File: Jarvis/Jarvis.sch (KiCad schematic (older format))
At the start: 180 parts, among them IC1 ADP1607, IC2 MAX-8Q, IC3 MPU-9250, IC4 STM32F411CxUx, IC5 Si4460, IC6 MS5611-01BA03, IC7 S25FL127S, J1 PYRO, J2 PWR, J3 ARM, J4 MICROUSB, P1 SMA, P2 SMA, P3 SWD_TC, Q1 PFET, Q2 PFET, Q3 PFET, Q4 NFET, Q5 NFET, Q6 NFET, Q7 NFET, X1 434MHz ANT, X10 Housing x1, X11 Housing x3, X12 M Crimps x6, X13 F Crimps x17, X14 Crimp Tool, X15 RF Frame, X16 RF Cover, X2 Red LED, X3 AA Battery, X4 AA Holder, X5 ARM Switch, X6 Wire, X7 Heat Shrink, X8 Housing x1, X9 Housing x4, Y1 26MHz, Y2 30MHz

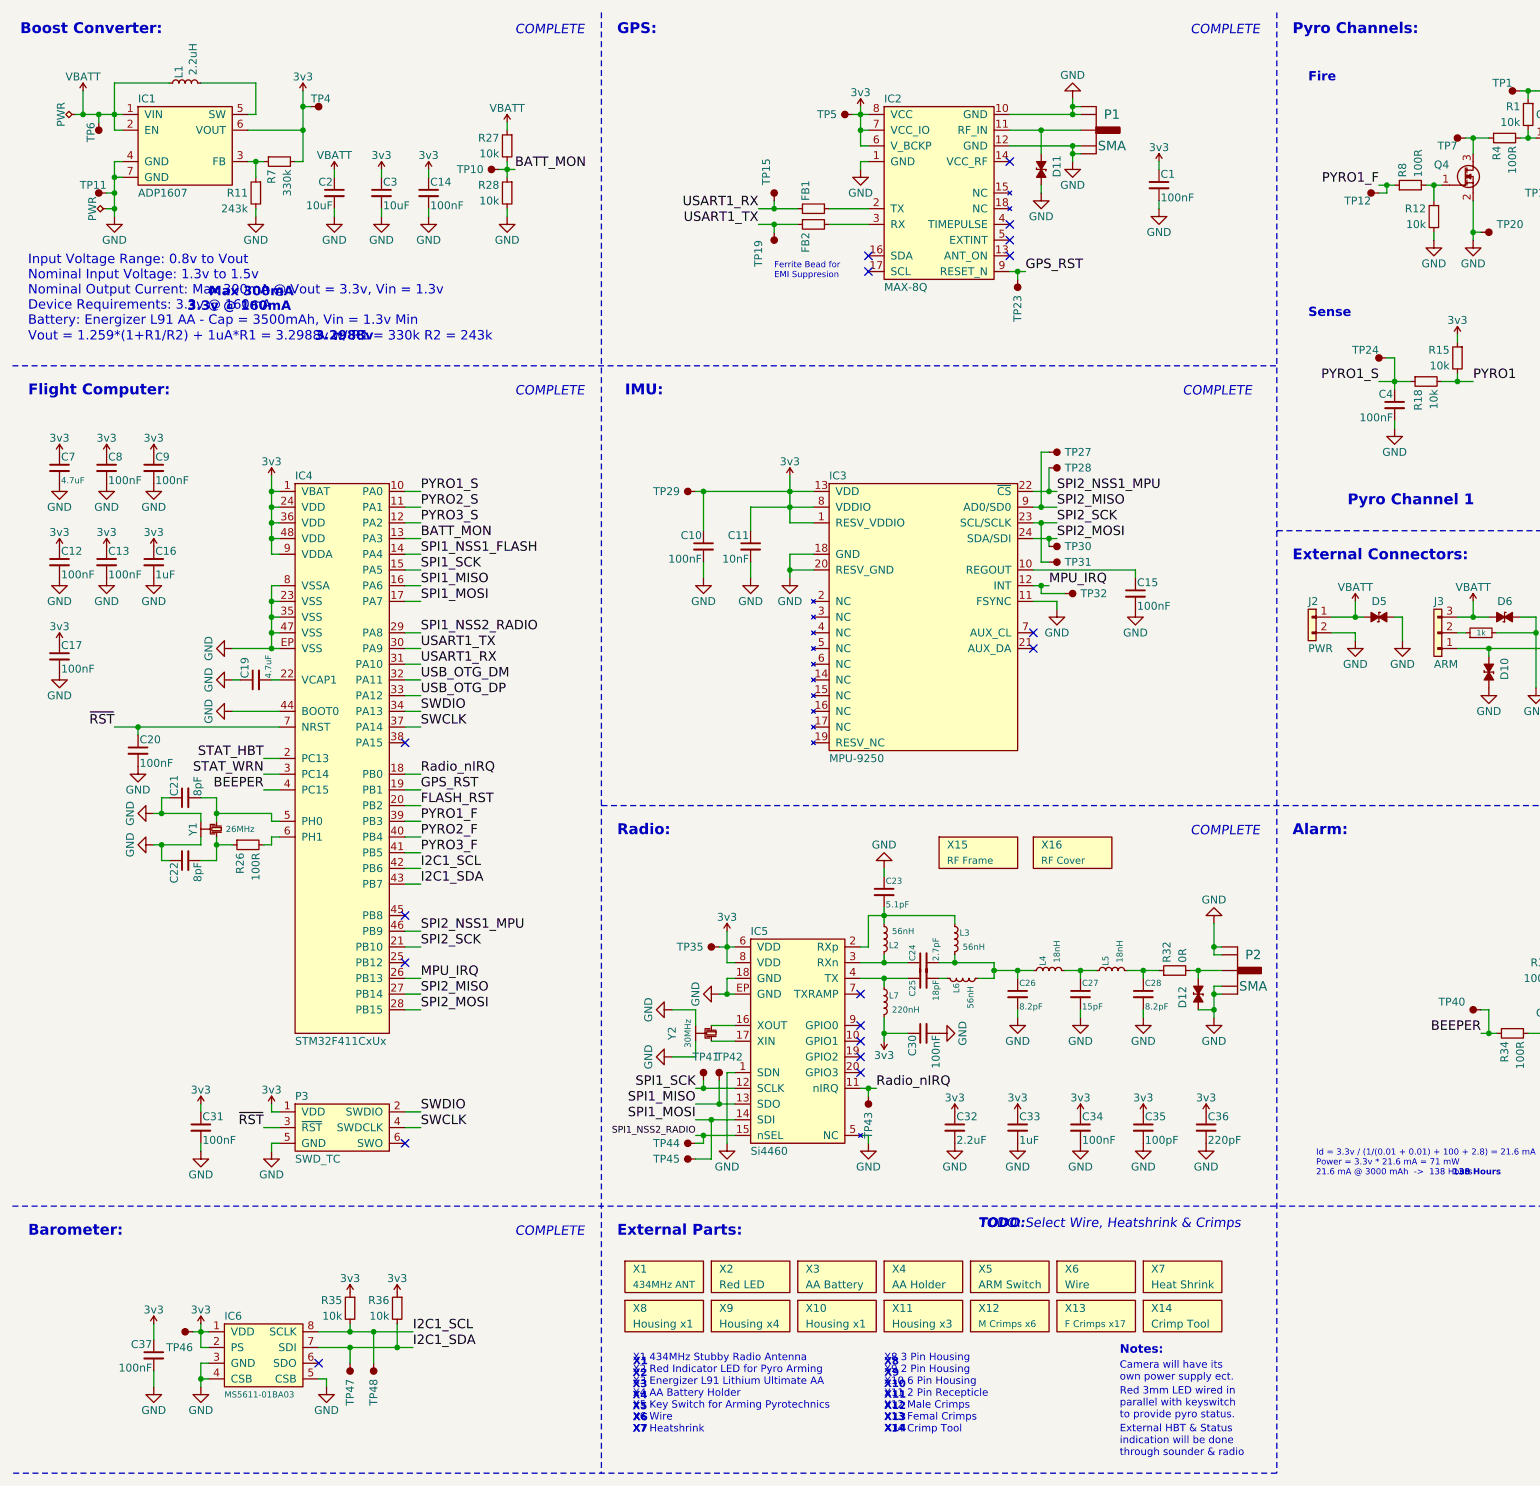
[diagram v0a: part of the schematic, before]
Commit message: Checked all Footprints
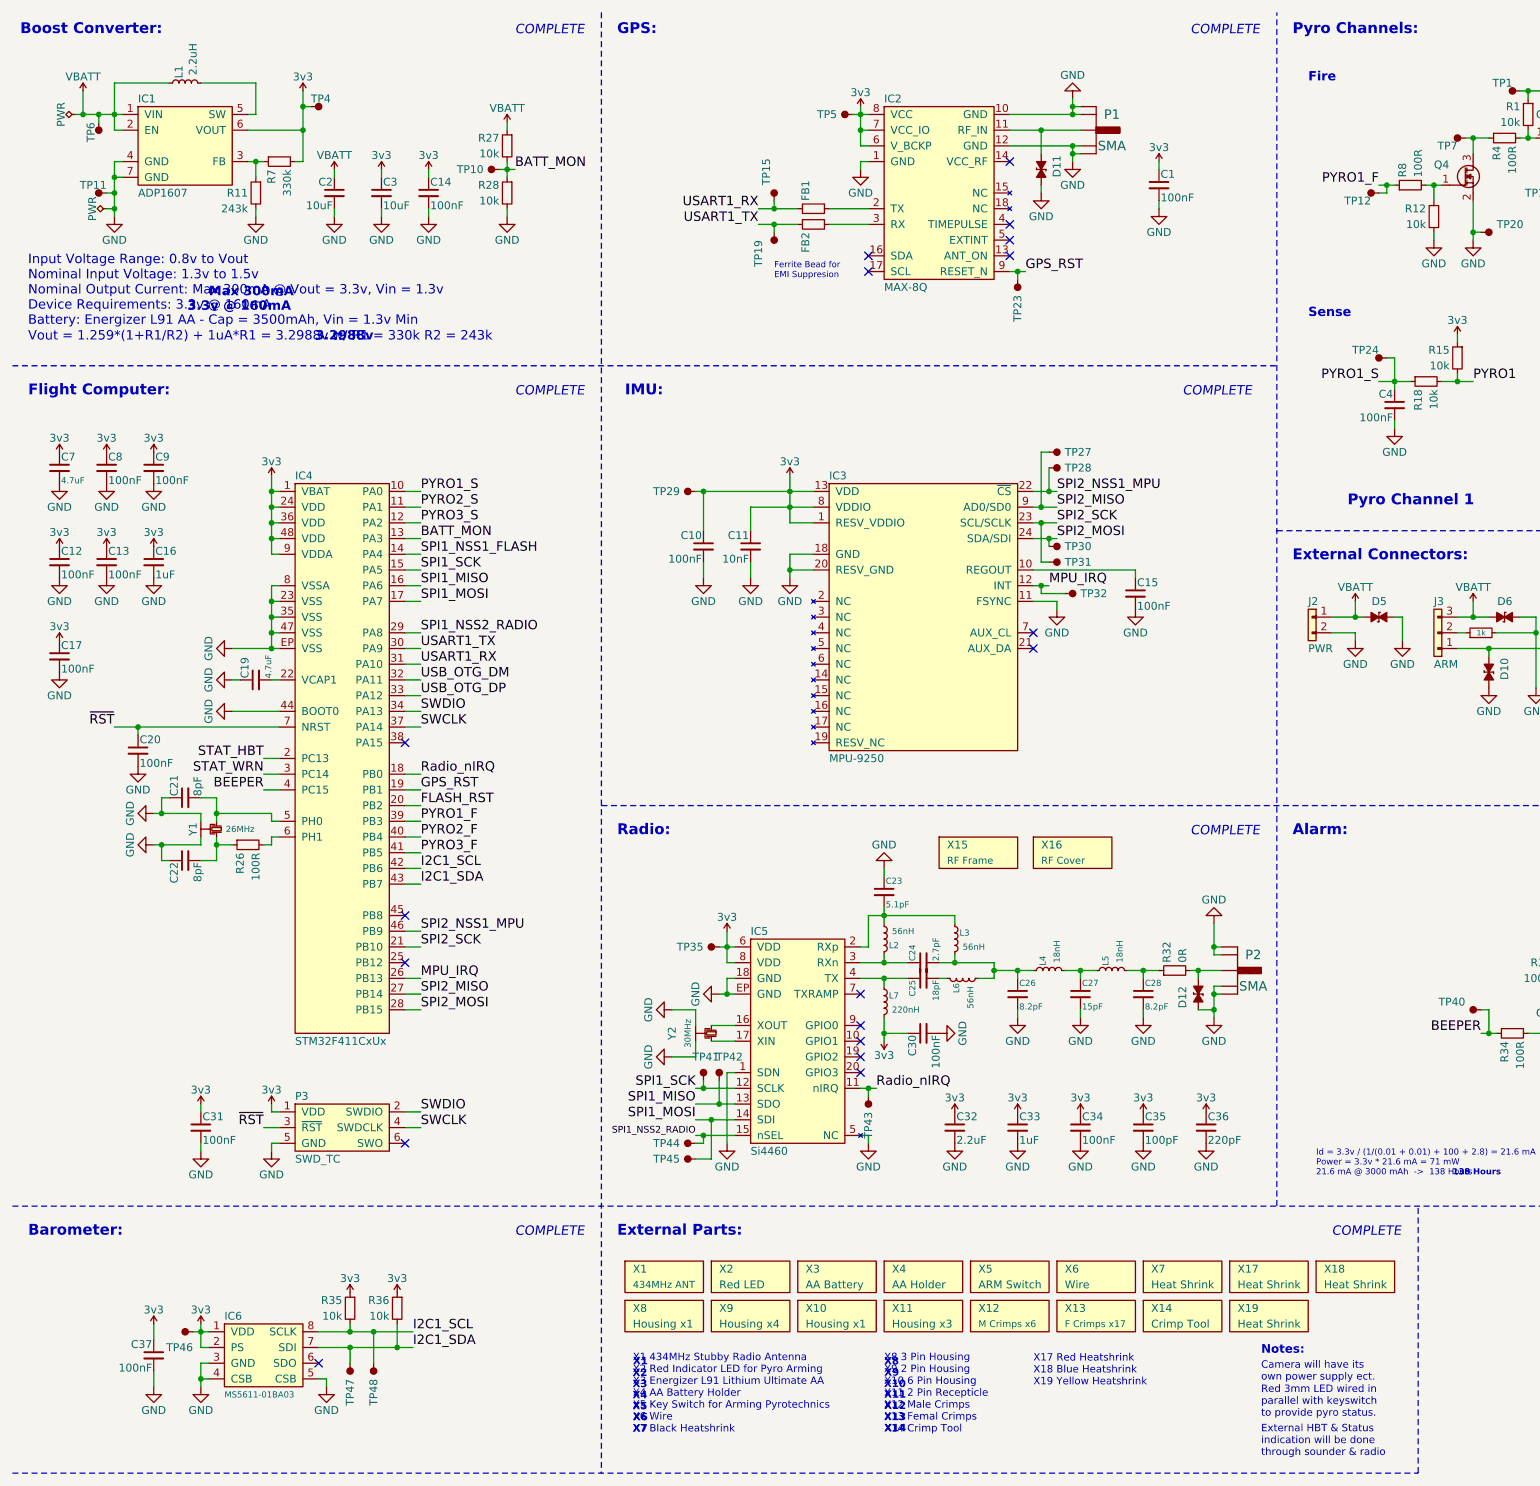
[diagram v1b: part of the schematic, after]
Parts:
- added X17, X18, X19: Heat Shrink, symbol PART
- C11: Farnell 2524673 -> 1414575
- C27: Farnell 1973025 -> 2496795
- D1, D2, D3: Farnell 1226372 -> 1328306
- D4: Farnell 1226390 -> 1328309
- IC7: footprint agg:WND008 -> agg:S25FL127S
- L1: footprint Inductors_NEOSID:Neosid_Inductor_SM-NE29_SMD1008 -> Library:VLF252012MT
- P2: Farnell 1608592 -> 1019325
- R10, R26, R29, R33, R34, R4, R5, R6, R8, R9: Farnell 1358015 -> 2072515
- X12: Farnell (none) -> 1830754
- X13: RS (none) -> 688-1381
- X6: Farnell (none) -> 2367724
- X7: Farnell (none) -> 1210349
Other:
- note added: "X1 434MHz Stubby Radio Antenna\nX2 Red Indicator LED for Pyro Arming\nX3 Energizer L91 Lithium Ultimate AA\nX4 AA Battery Holder\nX5 Key Switch for Arming Pyrotechnics\nX6 Wire\nX7 Black Heatshrink"
- note added: "X17 Red Heatshrink\nX18 Blue Heatshrink\nX19 Yellow Heatshrink"
- note removed: "TODO:"
- note removed: "TODO: Select Wire, Heatshrink & Crimps"
- note removed: "X1 434MHz Stubby Radio Antenna\nX2 Red Indicator LED for Pyro Arming\nX3 Energizer L91 Lithium Ultimate AA\nX4 AA Battery Holder\nX5 Key Switch for Arming Pyrotechnics\nX6 Wire\nX7 Heatshrink"
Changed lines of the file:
@@
 F 0 "L1" H 1630 990 50  0000 L CNN
 F 1 "2.2uH" H 1650 900 50  0000 L CNN
-F 2 "Inductors_NEOSID:Neosid_Inductor_SM-NE29_SMD1008" H 1600 950 50  0001 C CNN
+F 2 "Library:VLF252012MT" H 1600 950 50  0001 C CNN
 F 3 "http://www.farnell.com/datasheets/1759590.pdf" H 1600 950 50  0001 C CNN
 F 4 "2455292" H 1600 950 60  0001 C CNN "Farnell"
@@
 F 2 "agg:0402-L" H 2000 5800 50  0001 C CNN
 F 3 "http://www.farnell.com/datasheets/1729045.pdf" H 2000 5800 50  0001 C CNN
-F 4 "1358015" H 2000 5800 60  0001 C CNN "Farnell"
+F 4 "2072515" H 2000 5800 60  0001 C CNN "Farnell"
 	1    2000 5800
 	0    -1   1    0
@@
 Text Label 11700 4750 0    60   ~ 0
 PYRO3
-Text Notes 7550 9220 0    47   ~ 0
+Text Notes 8450 9220 0    47   ~ 0
 Camera will have its\nown power supply ect.
 $Comp
@@
 F 2 "agg:0603-LED" H 12650 4800 50  0001 C CNN
 F 3 "http://www.farnell.com/datasheets/1693302.pdf" H 12650 4800 50  0001 C CNN
-F 4 "1226372" H 12650 4800 60  0001 C CNN "Farnell"
+F 4 "1328306" H 12650 4800 60  0001 C CNN "Farnell"
 	1    12650 4800
 	0    -1   -1   0
@@
 F 2 "agg:0603-LED" H 15000 4800 50  0001 C CNN
 F 3 "http://www.farnell.com/datasheets/302470.pdf" H 15000 4800 50  0001 C CNN
-F 4 "1226390" H 15000 4800 60  0001 C CNN "Farnell"
+F 4 "1328309" H 15000 4800 60  0001 C CNN "Farnell"
 	1    15000 4800
 	0    -1   -1   0
@@
 F 2 "agg:0402-L" H 7300 6750 50  0001 C CNN
 F 3 "http://www.farnell.com/datasheets/1446011.pdf" H 7300 6750 50  0001 C CNN
-F 4 "1973025" H 7300 6750 60  0001 C CNN "Farnell"
+F 4 "2496795" H 7300 6750 60  0001 C CNN "Farnell"
 	1    7300 6750
 	1    0    0    -1
@@
 F 2 "Library:SMA-142-0701-801" H 8300 6600 60  0001 C CNN
 F 3 "http://www.farnell.com/datasheets/493539.pdf" H 8300 6600 60  0001 C CNN
-F 4 "1608592" H 8300 6600 60  0001 C CNN "Farnell"
+F 4 "1019325" H 8300 6600 60  0001 C CNN "Farnell"
 	1    8300 6600
 	1    0    0    1
@@
 F 2 "agg:0402-L" H 5200 3900 50  0001 C CNN
 F 3 "http://www.farnell.com/datasheets/2009679.pdf" H 5200 3900 50  0001 C CNN
-F 4 "2524673" H 5200 3900 60  0001 C CNN "Farnell"
+F 4 "1414575" H 5200 3900 60  0001 C CNN "Farnell"
 	1    5200 3900
 	-1   0    0    -1
@@
 F 2 "agg:0402-L" H 10050 7000 50  0001 C CNN
 F 3 "http://www.farnell.com/datasheets/1729045.pdf" H 10050 7000 50  0001 C CNN
-F 4 "1358015" H 10050 7000 60  0001 C CNN "Farnell"
+F 4 "2072515" H 10050 7000 60  0001 C CNN "Farnell"
 	1    10050 7000
 	0    -1   1    0
@@
 F 2 "agg:0402-L" H 10350 6600 50  0001 C CNN
 F 3 "http://www.farnell.com/datasheets/1729045.pdf" H 10350 6600 50  0001 C CNN
-F 4 "1358015" H 10350 6600 60  0001 C CNN "Farnell"
+F 4 "2072515" H 10350 6600 60  0001 C CNN "Farnell"
 	1    10350 6600
 	-1   0    0    -1
@@
 F 2 "agg:0603-LED" H 13450 4800 50  0001 C CNN
 F 3 "http://www.farnell.com/datasheets/1693302.pdf" H 13450 4800 50  0001 C CNN
-F 4 "1226372" H 13450 4800 60  0001 C CNN "Farnell"
+F 4 "1328306" H 13450 4800 60  0001 C CNN "Farnell"
 	1    13450 4800
 	0    -1   -1   0
@@
 F 2 "agg:0603-LED" H 14200 4800 50  0001 C CNN
 F 3 "http://www.farnell.com/datasheets/1693302.pdf" H 14200 4800 50  0001 C CNN
-F 4 "1226372" H 14200 4800 60  0001 C CNN "Farnell"
+F 4 "1328306" H 14200 4800 60  0001 C CNN "Farnell"
 	1    14200 4800
 	0    -1   -1   0
@@
 F 2 "agg:0402-L" H 9400 1600 50  0001 C CNN
 F 3 "http://www.farnell.com/datasheets/1729045.pdf" H 9400 1600 50  0001 C CNN
-F 4 "1358015" H 9400 1600 60  0001 C CNN "Farnell"
+F 4 "2072515" H 9400 1600 60  0001 C CNN "Farnell"
 	1    9400 1600
 	0    -1   -1   0
@@
 F 2 "agg:0402-L" H 11850 1600 50  0001 C CNN
 F 3 "http://www.farnell.com/datasheets/1729045.pdf" H 11850 1600 50  0001 C CNN
-F 4 "1358015" H 11850 1600 60  0001 C CNN "Farnell"
+F 4 "2072515" H 11850 1600 60  0001 C CNN "Farnell"
 	1    11850 1600
 	0    -1   -1   0
@@
 F 2 "agg:0402-L" H 14300 1600 50  0001 C CNN
 F 3 "http://www.farnell.com/datasheets/1729045.pdf" H 14300 1600 50  0001 C CNN
-F 4 "1358015" H 14300 1600 60  0001 C CNN "Farnell"
+F 4 "2072515" H 14300 1600 60  0001 C CNN "Farnell"
 	1    14300 1600
 	0    -1   -1   0
@@
 F 2 "agg:0402-L" H 14900 1300 50  0001 C CNN
 F 3 "http://www.farnell.com/datasheets/1729045.pdf" H 14900 1300 50  0001 C CNN
-F 4 "1358015" H 14900 1300 60  0001 C CNN "Farnell"
+F 4 "2072515" H 14900 1300 60  0001 C CNN "Farnell"
 	1    14900 1300
 	0    -1   1    0
@@
 F 2 "agg:0402-L" H 12450 1300 50  0001 C CNN
 F 3 "http://www.farnell.com/datasheets/1729045.pdf" H 12450 1300 50  0001 C CNN
-F 4 "1358015" H 12450 1300 60  0001 C CNN "Farnell"
+F 4 "2072515" H 12450 1300 60  0001 C CNN "Farnell"
 	1    12450 1300
 	0    -1   1    0
@@
 F 2 "agg:0402-L" H 10000 1300 50  0001 C CNN
 F 3 "http://www.farnell.com/datasheets/1729045.pdf" H 10000 1300 50  0001 C CNN
-F 4 "1358015" H 10000 1300 60  0001 C CNN "Farnell"
+F 4 "2072515" H 10000 1300 60  0001 C CNN "Farnell"
 	1    10000 1300
 	0    -1   1    0
@@
 	1    0    0    -1
 $EndComp
-Text Notes 7550 9460 0    47   ~ 0
+Text Notes 8450 9450 0    47   ~ 0
 Red 3mm LED wired in\nparallel with keyswitch\nto provide pyro status.
 Text Notes 4450 9550 0    47   ~ 0
-X1 434MHz Stubby Radio Antenna\nX2 Red Indicator LED for Pyro Arming\nX3 Energizer L91 Lithium Ultimate AA\nX4 AA Battery Holder\nX5 Key Switch for Arming Pyrotechnics\nX6 Wire\nX7 Heatshrink
+X1 434MHz Stubby Radio Antenna\nX2 Red Indicator LED for Pyro Arming\nX3 Energizer L91 Lithium Ultimate AA\nX4 AA Battery Holder\nX5 Key Switch for Arming Pyrotechnics\nX6 Wire\nX7 Black Heatshrink
 $Comp
 L CONN_01x03 J3
@@
 	0    -1   -1   0
 $EndComp
-Text Notes 7550 9050 0    55   ~ 11
+Text Notes 8450 9050 0    55   ~ 11
 Notes:
-Text Notes 7550 9700 0    47   ~ 0
+Text Notes 8450 9700 0    47   ~ 0
 External HBT & Status\nindication will be done\nthrough sounder & radio
 Text Notes 4451 9122 0    47   ~ 9
@@
 F 2 "" H 7150 8850 50  0001 C CNN
 F 3 "http://www.farnell.com/datasheets/621888.pdf" H 7150 8850 50  0001 C CNN
+F 4 "688-1381" H 7150 8850 60  0001 C CNN "RS"
 	1    7150 8850
 	1    0    0    -1
@@
 F 2 "" H 7150 8600 50  0001 C CNN
 F 3 "" H 7150 8600 50  0001 C CNN
+F 4 "2367724" H 7150 8600 60  0001 C CNN "Farnell"
 	1    7150 8600
 	1    0    0    -1
@@
 F 2 "" H 6600 8850 50  0001 C CNN
 F 3 "" H 6600 8850 50  0001 C CNN
+F 4 "1830754" H 6600 8850 60  0001 C CNN "Farnell"
 	1    6600 8850
 	1    0    0    -1
@@
 F 2 "" H 7700 8600 50  0001 C CNN
 F 3 "" H 7700 8600 50  0001 C CNN
+F 4 "1210349" H 7700 8600 60  0001 C CNN "Farnell"
 	1    7700 8600
 	1    0    0    -1
@@
 Text Notes 6051 9549 0    47   ~ 9
 X14
-Text Notes 6650 8250 0    60   Italic 0
-TODO: Select Wire, Heatshrink & Crimps
 $Comp
 L GND #PWR0101
@@
 	1    0    0    -1
 $EndComp
-Text Notes 6650 8250 0    60   Italic 12
-TODO:
 $Comp
 L ESD_DIODE D5
@@
 F 0 "IC7" H 14750 6900 50  0000 L CNN
 F 1 "S25FL127S" H 14750 6300 50  0000 L CNN
-F 2 "agg:WND008" H 14750 6200 50  0001 L CNN
+F 2 "agg:S25FL127S" H 14750 6200 50  0001 L CNN
 F 3 "https://www.spansion.com/Support/Datasheets/S25FL127S_00.pdf" H 14750 6100 50  0001 L CNN
 F 4 "2328003" H 14750 6000 50  0001 L CNN "Farnell"
@@
 F 2 "agg:0402-L" H 10550 6600 50  0001 C CNN
 F 3 "http://www.farnell.com/datasheets/1729045.pdf" H 10550 6600 50  0001 C CNN
-F 4 "1358015" H 10550 6600 60  0001 C CNN "Farnell"
+F 4 "2072515" H 10550 6600 60  0001 C CNN "Farnell"
 	1    10550 6600
 	1    0    0    -1
@@
 	11150 4450 11150 5000
 Wire Notes Line
-	8550 9800 500  9800
+	500  9800 9450 9800
 Wire Notes Line
 	4250 500  4250 9800
@@
 Wire Wire Line
 	1800 5600 2150 5600
-Wire Notes Line
-	8550 500  8550 9800
 Wire Wire Line
 	5950 7650 5950 7700
@@
 	1    0    0    -1
 $EndComp
+$Comp
+L PART X17
+U 1 1 571ECFBC
+P 8250 8600
+F 0 "X17" H 8300 8700 50  0000 L CNN
+F 1 "Heat Shrink" H 8300 8600 50  0000 L CNN
+F 2 "" H 8250 8600 50  0001 C CNN
+F 3 "" H 8250 8600 50  0001 C CNN
+F 4 "1210365" H 8250 8600 60  0001 C CNN "Farnell"
+	1    8250 8600
+	1    0    0    -1
+$EndComp
+$Comp
+L PART X18
+U 1 1 571ED208
+P 8800 8600
+F 0 "X18" H 8850 8700 50  0000 L CNN
+F 1 "Heat Shrink" H 8850 8600 50  0000 L CNN
+F 2 "" H 8800 8600 50  0001 C CNN
+F 3 "" H 8800 8600 50  0001 C CNN
+F 4 " 1210405" H 8800 8600 60  0001 C CNN "Farnell"
+	1    8800 8600
+	1    0    0    -1
+$EndComp
+$Comp
+L PART X19
+U 1 1 571ED451
+P 8250 8850
+F 0 "X19" H 8300 8950 50  0000 L CNN
+F 1 "Heat Shrink" H 8300 8850 50  0000 L CNN
+F 2 "" H 8250 8850 50  0001 C CNN
+F 3 "" H 8250 8850 50  0001 C CNN
+F 4 "1210381" H 8250 8850 60  0001 C CNN "Farnell"
+	1    8250 8850
+	1    0    0    -1
+$EndComp
+Wire Notes Line
+	8550 8100 8550 500
+Wire Notes Line
+	9450 9800 9450 8100
+Text Notes 8900 8300 0    60   Italic 0
+COMPLETE
+Text Notes 7000 9250 0    47   ~ 0
+X17 Red Heatshrink\nX18 Blue Heatshrink\nX19 Yellow Heatshrink
 $EndSCHEMATC
